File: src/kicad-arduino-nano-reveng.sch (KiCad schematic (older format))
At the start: 15 parts, among them J1 USB_B_Mini, U1 ATmega328P-AU

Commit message: Wiring
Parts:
- added C1, C6: CP, Capacitor_Tantalum_SMD:CP_EIA-3216-10_Kemet-I, symbol Device:CP
- added C2, C3, C4, C5, C7: C, Capacitor_SMD:C_0603_1608Metric, symbol Device:C
- added D5: D_Schottky, Diode_SMD:D_SOD-123, symbol Device:D_Schottky
- added R1: 103, Resistor_SMD:R_0603_1608Metric, symbol Device:R
- added R2, R3: R, Resistor_SMD:R_0603_1608Metric, symbol Device:R
- added U1: AMS1117-5.0, Package_TO_SOT_SMD:SOT-223, symbol Regulator_Linear:AMS1117-5.0
- added U3: CH340G, Package_SO:SOIC-16_3.9x9.9mm_P1.27mm, symbol Interface_USB:CH340G
- added Y2: Crystal, Crystal:Crystal_SMD_MicroCrystal_CC7V-T1A-2Pin_3.2x1.5mm, symbol Device:Crystal
- D1: renamed from D?; value LED_ALT -> RX; footprint (none) -> LED_SMD:LED_0603_1608Metric_Pad1.05x0.95mm_HandSolder
- D2: renamed from D?; value LED_ALT -> TX; footprint (none) -> LED_SMD:LED_0603_1608Metric_Pad1.05x0.95mm_HandSolder
- D3: renamed from D?; value LED_ALT -> PWR; footprint (none) -> LED_SMD:LED_0603_1608Metric_Pad1.05x0.95mm_HandSolder
- D4: renamed from D?; value LED_ALT -> L; footprint (none) -> LED_SMD:LED_0603_1608Metric_Pad1.05x0.95mm_HandSolder
- J1: footprint (none) -> Connector_USB:USB_Mini-B_Lumberg_2486_01_Horizontal
- J2: renamed from J?; value Conn_02x03_Odd_Even -> ISP; footprint (none) -> Connector_PinHeader_2.54mm:PinHeader_2x03_P2.54mm_Vertical; symbol Connector_Generic:Conn_02x03_Odd_Even -> Connector:AVR-ISP-6
- J3: renamed from J?; footprint (none) -> Connector_PinHeader_2.54mm:PinHeader_1x15_P2.54mm_Vertical; symbol Connector_Generic:Conn_01x15 -> igorkelvin:Conn_Nano_01
- J4: renamed from J?; footprint (none) -> Connector_PinHeader_2.54mm:PinHeader_1x15_P2.54mm_Vertical; symbol Connector_Generic:Conn_01x15 -> igorkelvin:Conn_Nano_02
- R4, R5, R6, R7: renamed from R?; value R -> 102; footprint (none) -> Resistor_SMD:R_0603_1608Metric
- SW1: renamed from SW?; value SW_Push -> RESET; footprint (none) -> Button_Switch_SMD:SW_SPST_CK_RS282G05A3
- Y1: renamed from Y?; value Crystal -> Crystal_Atmega; footprint (none) -> Crystal:Crystal_SMD_3215-2Pin_3.2x1.5mm
- renumbered U1 to U2
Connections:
- net VUSB: now reaches J1.1 (VBUS)
- net VUSB: now also C6.1, C7.1, D5.2 (A)
- net D-: now reaches J1.2 (D-)
- net D-: now also U3.6 (UD-)
- net D+: now reaches J1.3 (D+)
- net D+: now also U3.5 (UD+)
- net GND: now reaches J1.5 (GND)
- net GND: now also D3.1 (K), D4.1 (K), J1.6 (Shield), J2.6 (GND), J3.4 (GND), J4.2 (GND), SW1.2, U2.21 (GND), U2.3 (GND), U2.5 (GND), C1.2, C2.2, C4.1, C5.1, C6.2, C7.2, U1.1 (GND), U3.1 (GND)
- net D3: now reaches U2.1 (PD3)
- net D3: now also J3.6 (D3)
- net D6: now reaches U2.10 (PD6)
- net D6: now also J3.9 (D6)
- net D7: now reaches U2.11 (PD7)
- net D7: now also J3.10 (D7)
- net D8: now reaches U2.12 (PB0)
- net D8: now also J3.11 (D8)
- net D9: now reaches U2.13 (PB1)
- net D9: now also J3.12 (D9)
- net D10: now reaches U2.14 (PB2)
- net D10: now also J3.13 (D10)
- net D11: now reaches U2.15 (PB3)
- net D11: now also J2.4 (MOSI), J3.14 (D11)
- net D12: now reaches U2.16 (PB4)
- net D12: now also J2.1 (MISO), J3.15 (D12)
- net D13: now reaches U2.17 (PB5)
- net D13: now also J2.3 (SCK), J4.15 (D13), R7.2
- net +5V: now reaches U2.18 (AVCC)
- net +5V: now also J2.2 (VCC), J4.4 (+5V), R4.2, R5.2, R6.2, U2.4 (VCC), U2.6 (VCC), C1.1, C2.1, D5.1 (K), R1.1, U1.2 (VO), U3.16 (VCC)
- net A6: now reaches U2.19 (ADC6)
- net A6: now also J4.6 (A6)
- net D4: now reaches U2.2 (PD4)
- net D4: now also J3.7 (D4)
- net AREF: now reaches U2.20 (AREF)
- net AREF: now also J4.13 (AREF), C4.2
- net A7: now reaches U2.22 (ADC7)
- net A7: now also J4.5 (A7)
- net A0: now reaches U2.23 (PC0)
- net A0: now also J4.12 (A0)
- net A1: now reaches U2.24 (PC1)
- net A1: now also J4.11 (A1)
- net A2: now reaches U2.25 (PC2)
- net A2: now also J4.10 (A2)
- net A3: now reaches U2.26 (PC3)
- net A3: now also J4.9 (A3)
- net A4: now reaches U2.27 (PC4)
- net A4: now also J4.8 (A4)
- net A5: now reaches U2.28 (PC5)
- net A5: now also J4.7 (A5)
- net RST: now reaches U2.29 (~RESET~/PC6)
- net RST: now also J2.5 (~RST), J3.3 (RST), J4.3 (RST), SW1.1, C3.1, R1.2
- net RX0: now reaches U2.30 (PD0)
- net RX0: now also D1.1 (K), J3.2 (RX0), R3.2
- net TX1: now reaches U2.31 (PD1)
- net TX1: now also D2.1 (K), J3.1 (TX1), R2.2
- net D2: now reaches U2.32 (PD2)
- net D2: now also J3.5 (D2)
- net XTAL1: now reaches U2.7 (XTAL1/PB6)
- net XTAL1: now also Y1.1
- net XTAL2: now reaches U2.8 (XTAL2/PB7)
- net XTAL2: now also Y1.2
- net D5: now reaches U2.9 (PD5)
- net D5: now also J3.8 (D5)
- net at R4.1: now also D1.2 (A)
- net at R5.1: now also D2.2 (A)
- net at R6.1: now also D3.2 (A)
- net at R7.1: now also D4.2 (A)
- net VIN: now reaches J4.1 (VIN)
- net VIN: now also U1.3 (VI)
- net 3V3: now reaches J4.14 (3V3)
- net 3V3: now also C5.2, U3.4 (V3)
- new net DTR: C3.2, U3.13 (~DTR)
- new net RXD: R2.1, U3.3 (RXD)
- new net TXD: R3.1, U3.2 (TXD)
- new net XI: U3.7 (XI), Y2.2
- new net XO: U3.8 (XO), Y2.1
- no-connect marks 0 -> 7
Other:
- moved on the sheet: J1, J3, J4, SW1

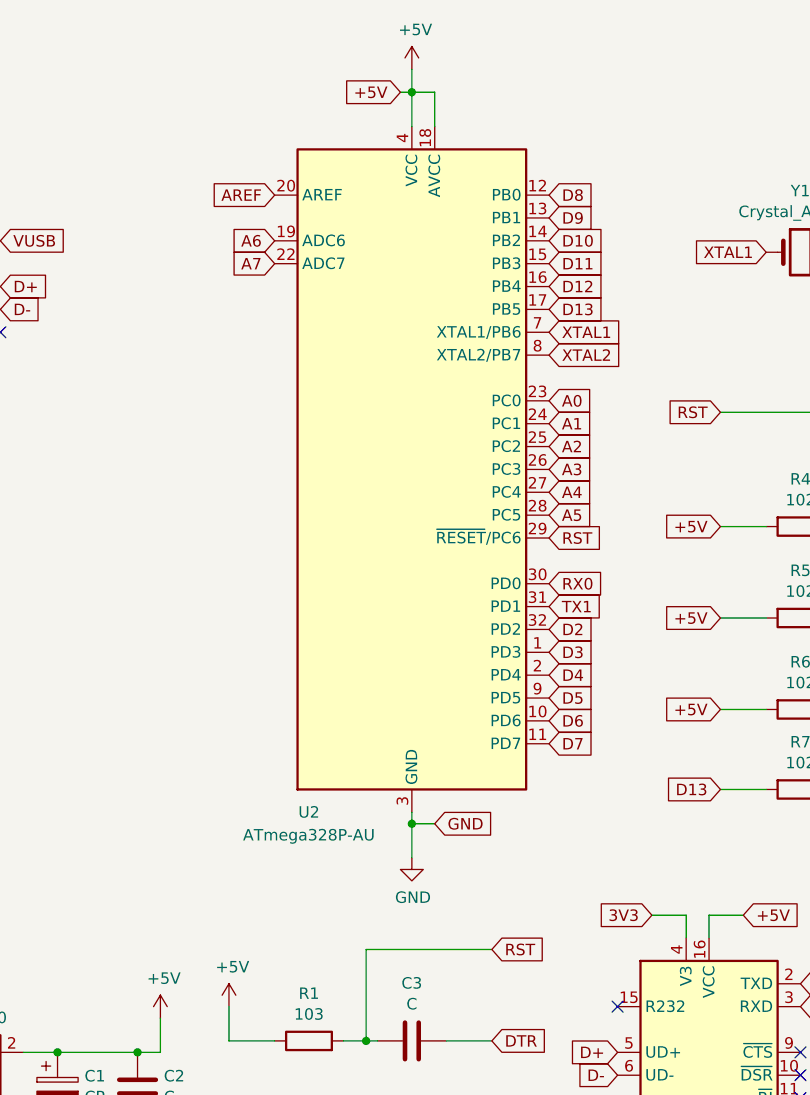
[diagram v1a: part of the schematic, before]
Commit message: Almost finishing routing
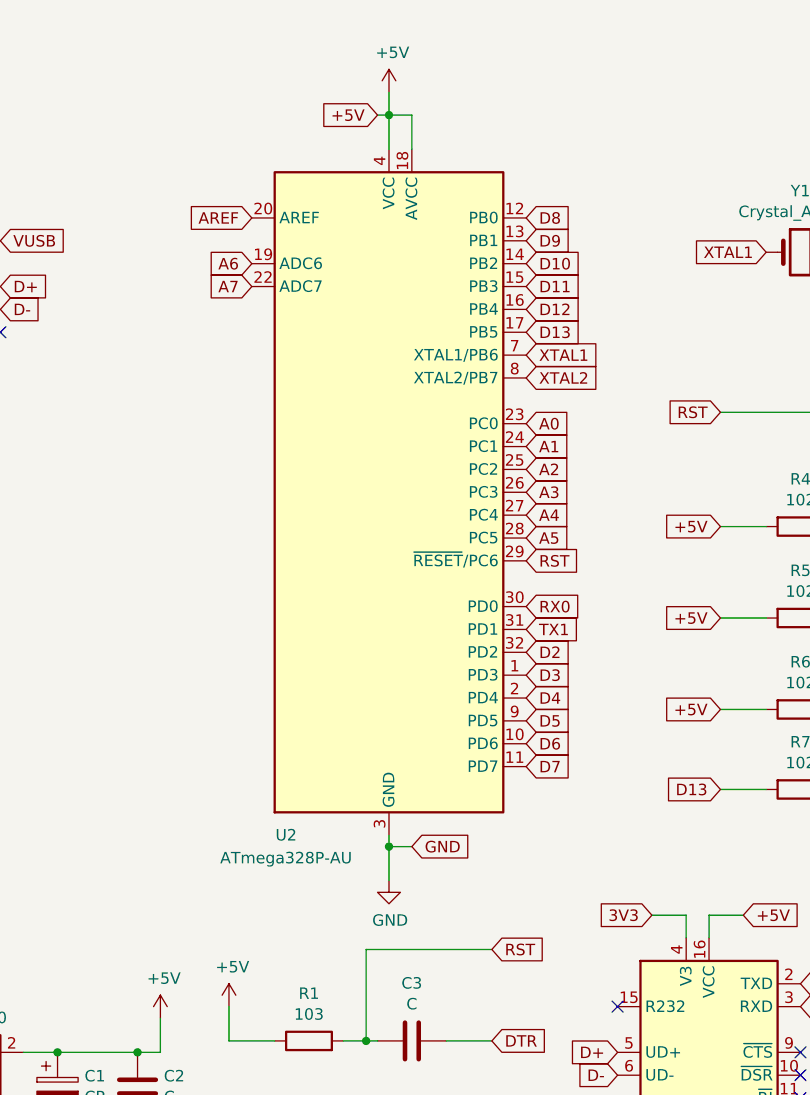
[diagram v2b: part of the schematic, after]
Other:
- moved on the sheet: U2
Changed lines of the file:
@@
 L MCU_Microchip_ATmega:ATmega328P-AU U2
 U 1 1 5F226888
-P 3250 2400
-F 0 "U2" H 2800 900 50  0000 C CNN
-F 1 "ATmega328P-AU" H 2800 800 50  0000 C CNN
-F 2 "Package_QFP:TQFP-32_7x7mm_P0.8mm" H 3250 2400 50  0001 C CIN
-F 3 "http://ww1.microchip.com/downloads/en/DeviceDoc/ATmega328_P%20AVR%20MCU%20with%20picoPower%20Technology%20Data%20Sheet%2040001984A.pdf" H 3250 2400 50  0001 C CNN
-	1    3250 2400
+P 3150 2500
+F 0 "U2" H 2700 1000 50  0000 C CNN
+F 1 "ATmega328P-AU" H 2700 900 50  0000 C CNN
+F 2 "Package_QFP:TQFP-32_7x7mm_P0.8mm" H 3150 2500 50  0001 C CIN
+F 3 "http://ww1.microchip.com/downloads/en/DeviceDoc/ATmega328_P%20AVR%20MCU%20with%20picoPower%20Technology%20Data%20Sheet%2040001984A.pdf" H 3150 2500 50  0001 C CNN
+	1    3150 2500
 	1    0    0    -1
 $EndComp
@@
 L power:GND #PWR08
 U 1 1 5F2B8802
-P 3250 4100
-F 0 "#PWR08" H 3250 3850 50  0001 C CNN
-F 1 "GND" H 3255 3927 50  0000 C CNN
-F 2 "" H 3250 4100 50  0001 C CNN
-F 3 "" H 3250 4100 50  0001 C CNN
-	1    3250 4100
-	1    0    0    -1
-$EndComp
-Wire Wire Line
-	3250 4100 3250 3950
-Wire Wire Line
-	3250 900  3250 750
-Wire Wire Line
-	3250 750  3200 750
-Text GLabel 3200 750  0    50   Input ~ 0
+P 3150 4200
+F 0 "#PWR08" H 3150 3950 50  0001 C CNN
+F 1 "GND" H 3155 4027 50  0000 C CNN
+F 2 "" H 3150 4200 50  0001 C CNN
+F 3 "" H 3150 4200 50  0001 C CNN
+	1    3150 4200
+	1    0    0    -1
+$EndComp
+Wire Wire Line
+	3150 4200 3150 4050
+Wire Wire Line
+	3150 1000 3150 850
+Wire Wire Line
+	3150 850  3100 850
+Text GLabel 3100 850  0    50   Input ~ 0
 +5V
 $Comp
 L power:+5V #PWR07
 U 1 1 5F2C2021
-P 3250 650
-F 0 "#PWR07" H 3250 500 50  0001 C CNN
-F 1 "+5V" H 3265 823 50  0000 C CNN
-F 2 "" H 3250 650 50  0001 C CNN
-F 3 "" H 3250 650 50  0001 C CNN
-	1    3250 650
-	1    0    0    -1
-$EndComp
-Wire Wire Line
-	3250 650  3250 750
-Connection ~ 3250 750
-Text GLabel 3350 3950 2    50   Input ~ 0
+P 3150 750
+F 0 "#PWR07" H 3150 600 50  0001 C CNN
+F 1 "+5V" H 3165 923 50  0000 C CNN
+F 2 "" H 3150 750 50  0001 C CNN
+F 3 "" H 3150 750 50  0001 C CNN
+	1    3150 750
+	1    0    0    -1
+$EndComp
+Wire Wire Line
+	3150 750  3150 850
+Connection ~ 3150 850
+Text GLabel 3250 4050 2    50   Input ~ 0
 GND
 Wire Wire Line
-	3250 3950 3350 3950
-Connection ~ 3250 3950
-Wire Wire Line
-	3250 3950 3250 3900
+	3150 4050 3250 4050
+Connection ~ 3150 4050
+Wire Wire Line
+	3150 4050 3150 4000
 Text GLabel 6850 2700 0    50   Input ~ 0
 GND
@@
 Text GLabel 6850 4000 0    50   Input ~ 0
 D13
-Text GLabel 3850 1700 2    50   Input ~ 0
+Text GLabel 3750 1800 2    50   Input ~ 0
 D13
 Text GLabel 4600 3800 0    50   Input ~ 0
@@
 Wire Wire Line
 	5450 2150 5900 2150
-Text GLabel 3850 2700 2    50   Input ~ 0
+Text GLabel 3750 2800 2    50   Input ~ 0
 RST
-Text GLabel 3850 2100 2    50   Input ~ 0
+Text GLabel 3750 2200 2    50   Input ~ 0
 A0
-Text GLabel 3850 2200 2    50   Input ~ 0
+Text GLabel 3750 2300 2    50   Input ~ 0
 A1
-Text GLabel 3850 2300 2    50   Input ~ 0
+Text GLabel 3750 2400 2    50   Input ~ 0
 A2
-Text GLabel 3850 2400 2    50   Input ~ 0
+Text GLabel 3750 2500 2    50   Input ~ 0
 A3
-Text GLabel 3850 2500 2    50   Input ~ 0
+Text GLabel 3750 2600 2    50   Input ~ 0
 A4
-Text GLabel 3850 2600 2    50   Input ~ 0
+Text GLabel 3750 2700 2    50   Input ~ 0
 A5
-Text GLabel 2650 1400 0    50   Input ~ 0
+Text GLabel 2550 1500 0    50   Input ~ 0
 A6
-Text GLabel 2650 1500 0    50   Input ~ 0
+Text GLabel 2550 1600 0    50   Input ~ 0
 A7
 Text GLabel 6850 3700 0    50   Input ~ 0
@@
 Text GLabel 6850 3000 0    50   Input ~ 0
 A7
-Text GLabel 2650 1200 0    50   Input ~ 0
+Text GLabel 2550 1300 0    50   Input ~ 0
 AREF
 Text GLabel 6850 3800 0    50   Input ~ 0
@@
 Text GLabel 5100 1450 2    50   Input ~ 0
 XTAL2
-Text GLabel 3850 1900 2    50   Input ~ 0
+Text GLabel 3750 2000 2    50   Input ~ 0
 XTAL2
-Text GLabel 3850 1800 2    50   Input ~ 0
+Text GLabel 3750 1900 2    50   Input ~ 0
 XTAL1
 Text GLabel 6300 1050 2    50   Input ~ 0
@@
 Text GLabel 6850 2150 0    50   Input ~ 0
 D11
-Text GLabel 3850 1600 2    50   Input ~ 0
+Text GLabel 3750 1700 2    50   Input ~ 0
 D12
-Text GLabel 3850 1500 2    50   Input ~ 0
+Text GLabel 3750 1600 2    50   Input ~ 0
 D11
-Text GLabel 3850 1400 2    50   Input ~ 0
+Text GLabel 3750 1500 2    50   Input ~ 0
 D10
-Text GLabel 3850 1300 2    50   Input ~ 0
+Text GLabel 3750 1400 2    50   Input ~ 0
 D9
-Text GLabel 3850 1200 2    50   Input ~ 0
+Text GLabel 3750 1300 2    50   Input ~ 0
 D8
 Text GLabel 6850 2050 0    50   Input ~ 0
@@
 Text GLabel 6850 1250 0    50   Input ~ 0
 D2
-Text GLabel 3850 3600 2    50   Input ~ 0
+Text GLabel 3750 3700 2    50   Input ~ 0
 D7
-Text GLabel 3850 3500 2    50   Input ~ 0
+Text GLabel 3750 3600 2    50   Input ~ 0
 D6
-Text GLabel 3850 3400 2    50   Input ~ 0
+Text GLabel 3750 3500 2    50   Input ~ 0
 D5
-Text GLabel 3850 3300 2    50   Input ~ 0
+Text GLabel 3750 3400 2    50   Input ~ 0
 D4
-Text GLabel 3850 3200 2    50   Input ~ 0
+Text GLabel 3750 3300 2    50   Input ~ 0
 D3
-Text GLabel 3850 3100 2    50   Input ~ 0
+Text GLabel 3750 3200 2    50   Input ~ 0
 D2
-Text GLabel 3850 3000 2    50   Input ~ 0
+Text GLabel 3750 3100 2    50   Input ~ 0
 TX1
-Text GLabel 3850 2900 2    50   Input ~ 0
+Text GLabel 3750 3000 2    50   Input ~ 0
 RX0
 Wire Wire Line
@@
 NoConn ~ 4950 4950
 Wire Wire Line
-	3350 900  3350 750
-Wire Wire Line
-	3350 750  3250 750
+	3250 1000 3250 850
+Wire Wire Line
+	3250 850  3150 850
 Text GLabel 4300 4350 0    50   Input ~ 0
 3V3

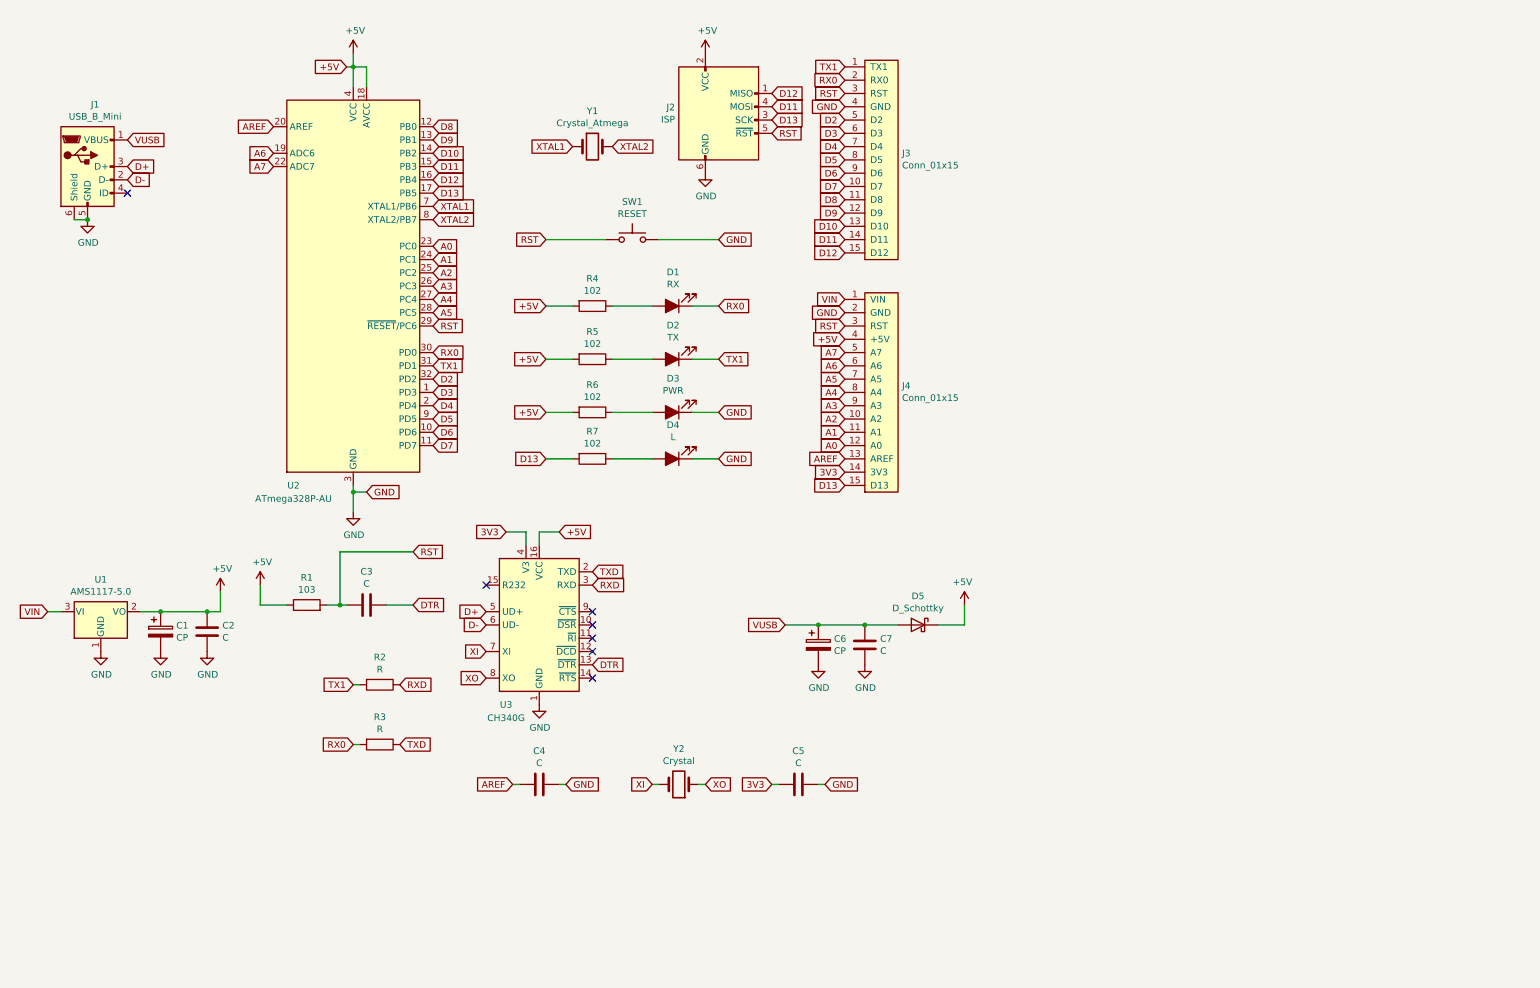
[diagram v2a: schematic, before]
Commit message: Rev 0
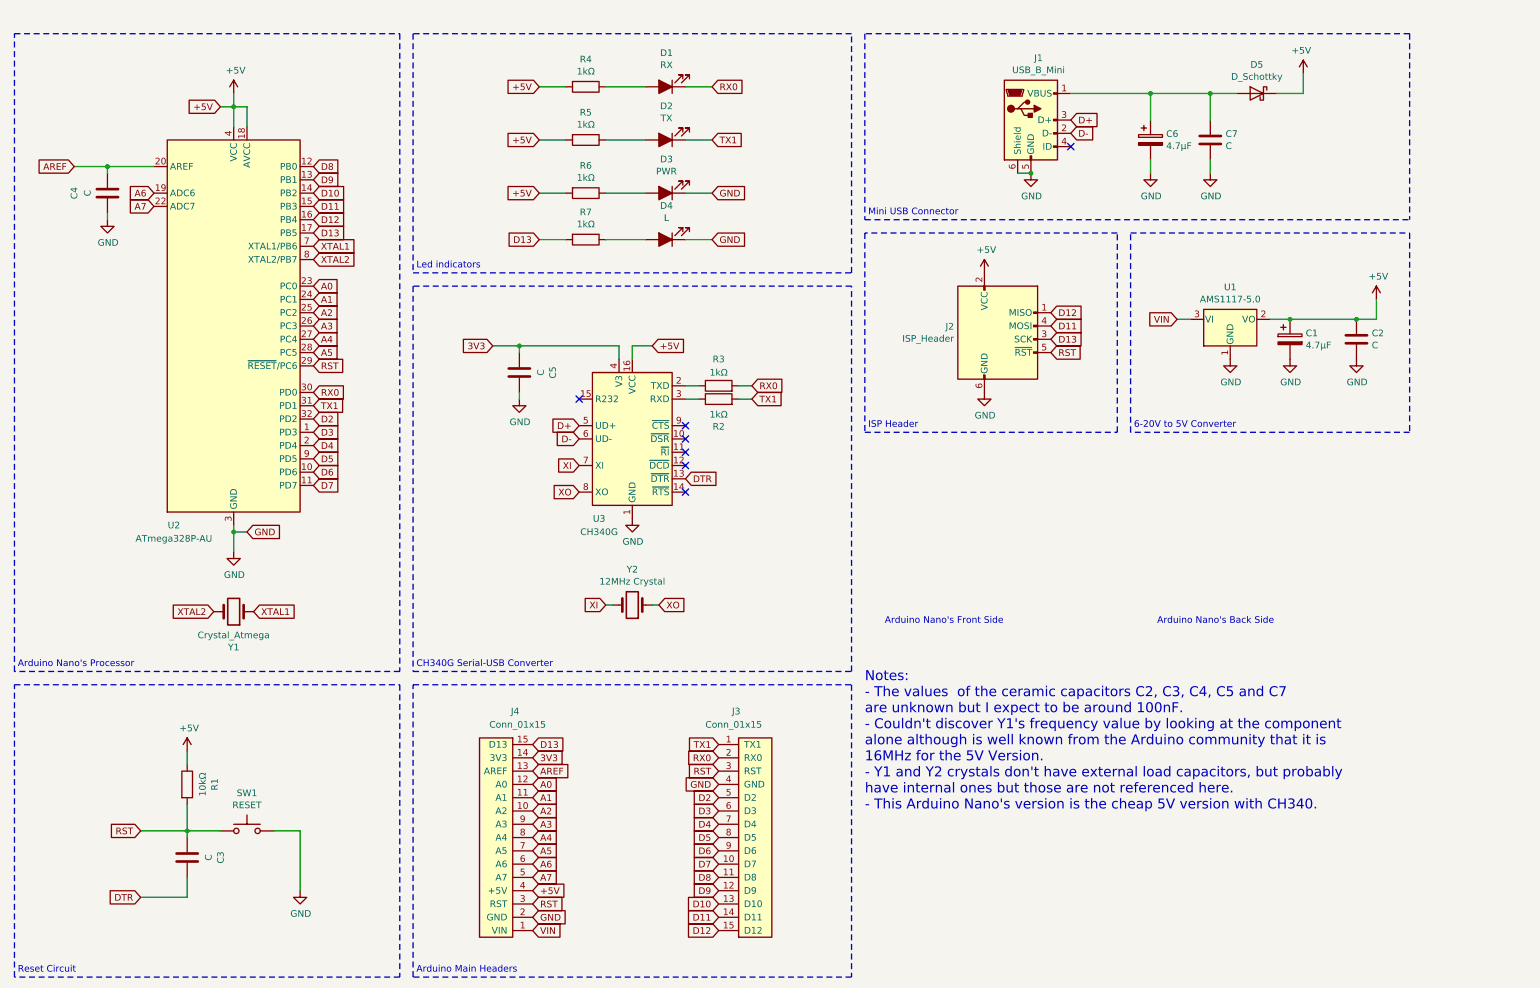
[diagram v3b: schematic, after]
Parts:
- C1, C6: value CP -> 4.7µF
- J2: value ISP -> ISP_Header
- R1: value 103 -> 10kΩ
- R2, R3: value R -> 1kΩ
- R4, R5, R6, R7: value 102 -> 1kΩ
- Y2: value Crystal -> 12MHz Crystal
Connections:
- net RXD: no longer names the net of R2.1, U3.3 (RXD)
- net TXD: no longer names the net of R3.1, U3.2 (TXD)
- net VUSB: no longer names the net of C6.1, C7.1, D5.2 (A), J1.1 (VBUS)
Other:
- note added: "6-20V to 5V Converter"
- note added: "Arduino Main Headers"
- note added: "Arduino Nano's Back Side"
- note added: "Arduino Nano's Front Side"
- note added: "Arduino Nano's Processor"
- note added: "CH340G Serial-USB Converter"
- note added: "ISP Header"
- note added: "Led indicators"
- note added: "Mini USB Connector"
- note added: "Notes:\n- The values of the ceramic capacitors C2, C3, C4, C5 and C7 \nare unknown but I expect to be around 100nF.\n- Couldn't discover Y1's frequency value by looking at the component \nalone although is well known from the Arduino community that it is \n16MHz for the 5V Version.\n- Y1 and Y2 crystals don't have external load capacitors, but probably\nhave internal ones but those are not refere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"
- note added: "Reset Circuit"
- moved on the sheet: C1, C2, C3, C4, C5, C6, C7, D1, D2, D3, D4, D5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
